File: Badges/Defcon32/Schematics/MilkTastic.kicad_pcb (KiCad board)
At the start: 2 copper layers, 7 x 7 mm, 34 parts, among them J1 2.8" Display, J2 SAO Conn, J3 Conn_01x04, J4 Conn_01x01, J5 XYAB, J7 Conn_01x01, J8 DPad, Q1 Q_NPN_BCE, SW1 LB, SW2 RB, SW7 Start/Sel, SW8 SW_SPDT, U1 MilkV Duo, U2 SK6812_Side, U3 SK6812_Side, U4 SK6812_Side, U5 SK6812_Side

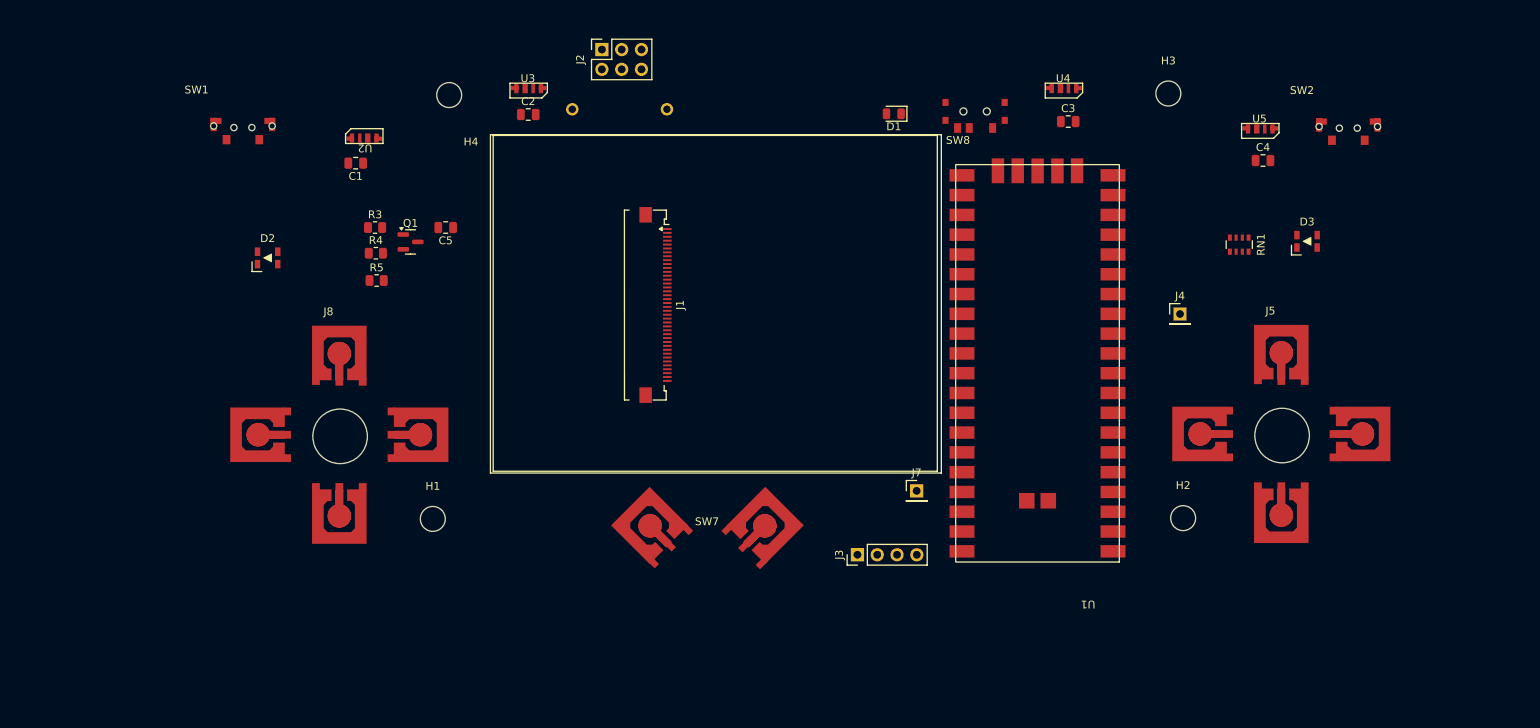
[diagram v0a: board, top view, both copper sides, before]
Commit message: Lets panel
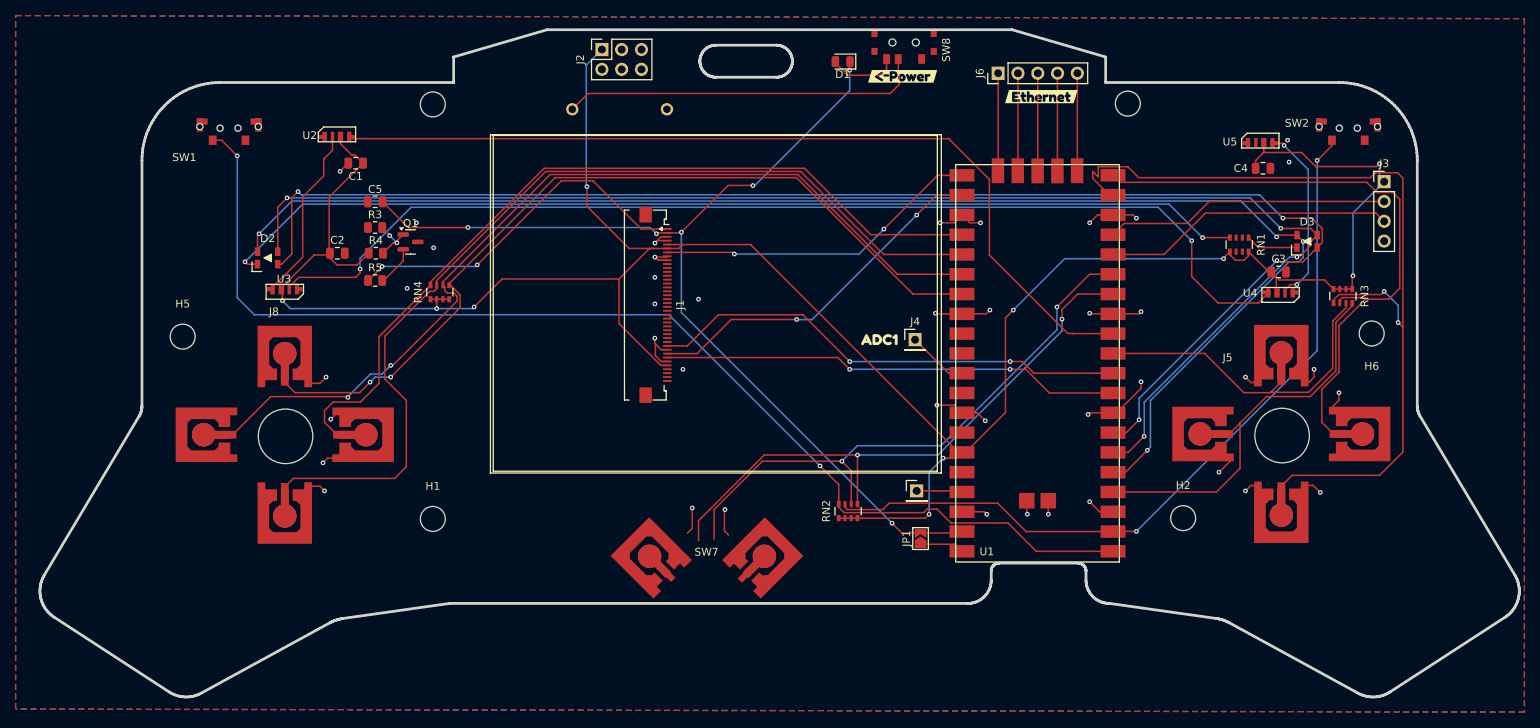
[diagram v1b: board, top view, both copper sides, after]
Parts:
- added H5: MountingHole, MountingHole:MountingHole_3.2mm_M3, F.Cu at (81.8, 62.8)
- added H6: MountingHole, MountingHole:MountingHole_3.2mm_M3, F.Cu at (234.4, 62.4)
- added J6: Ethernet, Connector_PinHeader_2.54mm:PinHeader_1x05_P2.54mm_Vertical, F.Cu at (186.5, 29.0)
- added JP1: USB_Pwr, Jumper:SolderJumper-2_P1.3mm_Open_TrianglePad1.0x1.5mm, F.Cu at (176.5, 88.7)
- added RN2: R_Pack04, Resistor_SMD:R_Array_Convex_4x0603, F.Cu at (167.2, 85.2)
- added RN3: R_Pack04, Resistor_SMD:R_Array_Convex_4x0603, F.Cu at (230.7, 57.6)
- added RN4: R_Pack04, Resistor_SMD:R_Array_Convex_4x0603, F.Cu at (114.8, 57.1)
- added kibuzzard-6692EF0B: G***, kibuzzard-6692EF0B, B.Cu at (232.0, 46.8)
- added kibuzzard-6692EF2E: G***, kibuzzard-6692EF2E, F.Cu at (171.2, 63.2)
- added kibuzzard-6692EF4B: G***, kibuzzard-6692EF4B, F.Cu at (192.0, 32.0)
- added kibuzzard-6692EF58: G***, kibuzzard-6692EF58, F.Cu at (174.2, 29.4)
- U2, U3, U4, U5: footprint UL_LED:SK6812SIDE-A-RVS -> UE_LED:SK6812SIDE-A-RVS
- moved J3 82.8 mm to (236.0, 42.9), turned to 0 degrees
- moved U3 40.6 mm to (94.8, 56.8)
- moved U4 38.2 mm to (222.6, 57.2)
- moved J4 34.2 mm to (175.8, 63.2)
- moved C3 33.2 mm to (222.4, 54.5)
- moved C2 30.3 mm to (101.7, 52.1)
- moved SW8 12.7 mm to (174.4, 25.1)
- moved C5 9.63 mm to (106.5, 45.5)
- moved D1 9.38 mm to (166.5, 27.5)
- moved J8 7.00 mm to (95.0, 75.6)
- moved H3 5.36 mm to (203.1, 32.9)
- moved SW7 3.91 mm to (149.0, 91.0)
- moved U2 3.51 mm to (101.7, 37.1)
- moved H4 2.42 mm to (113.9, 33.0)
- moved SW1 1.78 mm to (83.6, 34.8)
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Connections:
- C1 pad 1: A -> VCC
- C2 pad 1: A -> VCC
- C3 pad 1: A -> VCC
- C4 pad 1: A -> VCC
- D3 pad 1: R2 -> R1
- D3 pad 2: G2 -> G1
- D3 pad 4: B2 -> B1
- J1 pad 36: VDD -> VCC
- J1 pad 5: A -> VCC
- J1 pad 6: A -> VCC
- J2 pad 1: A -> VCC
- J3 pad 1: A -> VCC
- J5 pad 1: A -> Abtn
- R4 pad 1: A -> VCC
- RN1 pad 1: Net-(D2-A) -> Net-(D3-A)
- RN1 pad 4: Net-(D3-A) -> Net-(D2-A)
- RN1 pad 5: A -> VCC
- RN1 pad 8: A -> VCC
- U1 pad 1: R2 -> LeftBumper
- U1 pad 11: A -> Abtn
- U1 pad 2: G2 -> RightBumper
- U1 pad 24: B1 -> Right
- U1 pad 25: G1 -> Down
- U1 pad 26: R1 -> Left
- U1 pad 27: BV -> Up
- U1 pad 35: VDD -> VCC
- U1 pad 4: Up -> B
- U1 pad 40: unconnected-(U1-VBUS-Pad40) -> Net-(JP1-A)
- U1 pad 41: unconnected-(U1-TX+-Pad41) -> Net-(J6-Pin_1)
- U1 pad 42: unconnected-(U1-TX--Pad42) -> Net-(J6-Pin_2)
- U1 pad 43: VSS -> Net-(J6-Pin_3)
- U1 pad 44: unconnected-(U1-RX+-Pad44) -> Net-(J6-Pin_4)
- U1 pad 45: unconnected-(U1-RX--Pad45) -> Net-(J6-Pin_5)
- U1 pad 46: unconnected-(U1-USB_DM-Pad46) -> Net-(J9-Pin_2)
- U1 pad 47: unconnected-(U1-USB_DP-Pad47) -> Net-(J9-Pin_1)
- U1 pad 5: Left -> R1
- U1 pad 6: Down -> G1
- U1 pad 7: Right -> B1
- U2 pad 2: A -> VCC
- U3 pad 2: A -> VCC
- U4 pad 2: A -> VCC
- U5 pad 2: A -> VCC
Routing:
- net VCC: track 0.00 -> 321.5 mm, vias 0 -> 10
- net B1: track 0.00 -> 184.6 mm, vias 0 -> 4
- net G1: track 0.00 -> 182.2 mm, vias 0 -> 4
- net R1: track 0.00 -> 181.9 mm, vias 0 -> 4
- net LeftBumper: track 0.00 -> 150.1 mm, vias 0 -> 2
- net Net-(U3-Dout): track 0.00 -> 139.7 mm, vias 0 -> 2
- net Net-(D2-A): track 0.00 -> 133.0 mm, vias 0 -> 2
- net A: track 0.00 -> 131.1 mm, vias 0 -> 6
- net Down: track 0.00 -> 122.4 mm
- net Left: track 0.00 -> 117.4 mm, vias 0 -> 2
- net /SK6812: track 0.00 -> 113.9 mm
- net X: track 0.00 -> 112.4 mm, vias 0 -> 2
- net Up: track 0.00 -> 109.0 mm, vias 0 -> 2
- net Right: track 0.00 -> 105.7 mm
- net RightBumper: track 0.00 -> 100.4 mm, vias 0 -> 2
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- added copper zone on B.Cu, net VSS
- added copper zone on F.Cu, net VSS
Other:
- board size 7 x 7 mm -> 189.9 x 85.6 mm
